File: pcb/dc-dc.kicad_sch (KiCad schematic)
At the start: 30 parts

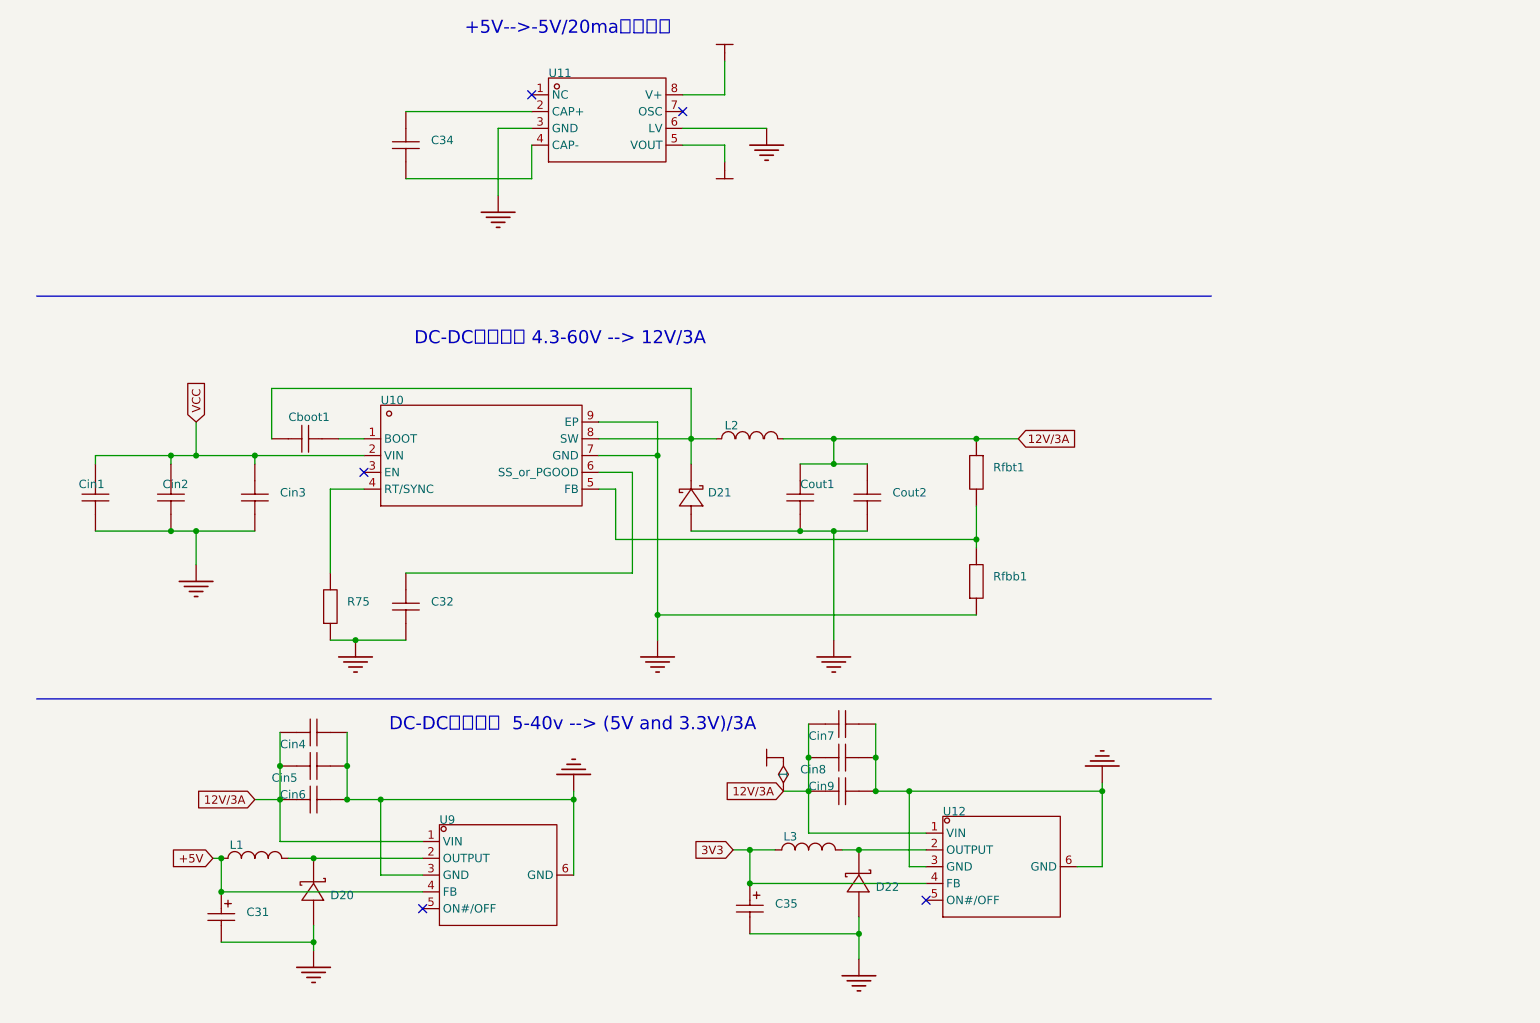
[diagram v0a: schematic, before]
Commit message: feat: update
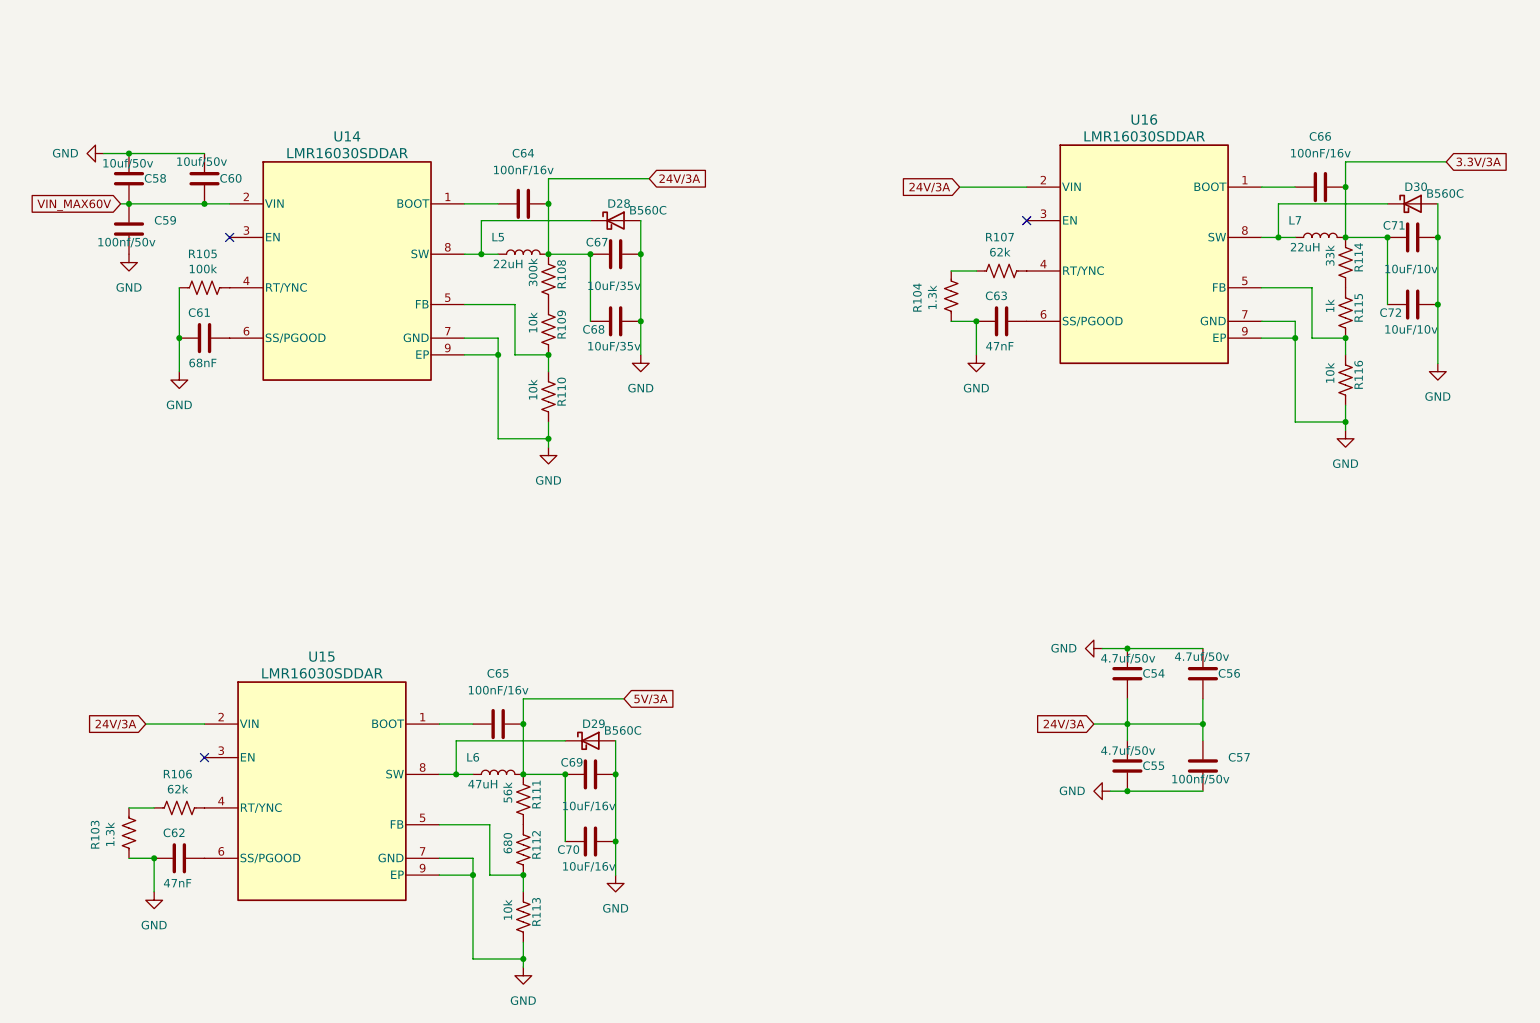
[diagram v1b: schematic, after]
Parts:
- removed 1: ~, ProDoc_CAN-easyedapro:, symbol ProDoc_CAN-easyedapro:Short-Symbol
- removed C31: 220uF, ProDoc_CAN-easyedapro:CASE-D_7343, symbol ProDoc_CAN-easyedapro:TAJD227K010RNJ
- removed C32: 33uF/25V, ProDoc_CAN-easyedapro:C0603, symbol ProDoc_CAN-easyedapro:CapAcitance
- removed C34: 47uF/25V, ProDoc_CAN-easyedapro:C0603, symbol ProDoc_CAN-easyedapro:CapAcitance
- removed C35: 330uF, ProDoc_CAN-easyedapro:CAP-SMD_L6.0-W3.2-R-RD, symbol ProDoc_CAN-easyedapro:TAJC337K006RNJ
- removed Cboot1: 0.1uF/50V, ProDoc_CAN-easyedapro:C0603, symbol ProDoc_CAN-easyedapro:CapAcitance
- removed Cin1, Cin6, Cin9: 0.1uF/100V, ProDoc_CAN-easyedapro:C0603, symbol ProDoc_CAN-easyedapro:CapAcitance
- removed Cin2, Cin3, Cin4, Cin5, Cin7, Cin8: 2.2uF/100V, ProDoc_CAN-easyedapro:C0603, symbol ProDoc_CAN-easyedapro:CapAcitance
- removed Cout1, Cout2: 47uF/50V, ProDoc_CAN-easyedapro:C0603, symbol ProDoc_CAN-easyedapro:CapAcitance
- removed D20, D22: ~, ProDoc_CAN-easyedapro:SMC_L7.5-W5.8-LS8.3-RD, symbol ProDoc_CAN-easyedapro:SS53C
- removed D21: ~, ProDoc_CAN-easyedapro:SMC_L6.9-W5.9-LS7.9-RD, symbol ProDoc_CAN-easyedapro:SS510SMC
- removed L1, L3: 33uH, ProDoc_CAN-easyedapro:IND-SMD_L11.5-W10.0_FXL1040, symbol ProDoc_CAN-easyedapro:FXL1040-330-M
- removed L2: 8.2uH, ProDoc_CAN-easyedapro:IND-SMD_L7.0-W6.6_FXL0630, symbol ProDoc_CAN-easyedapro:FXL0630-8R2-M
- removed R75: 50k, ProDoc_CAN-easyedapro:R0603, symbol ProDoc_CAN-easyedapro:电阻
- removed Rfbb1: 6.67k, ProDoc_CAN-easyedapro:R0603, symbol ProDoc_CAN-easyedapro:电阻
- removed Rfbt1: 100k, ProDoc_CAN-easyedapro:R0603, symbol ProDoc_CAN-easyedapro:电阻
- removed U10: ~, ProDoc_CAN-easyedapro:SO-8_L4.9-W3.9-P1.27-LS6.0-BL-EP, symbol ProDoc_CAN-easyedapro:LMR16030SDDAR
- removed U11: ~, ProDoc_CAN-easyedapro:SOP-8_L4.9-W3.9-P1.27-LS6.0-BL, symbol ProDoc_CAN-easyedapro:HT7660ARZ
- removed U12: ~, ProDoc_CAN-easyedapro:TO-263-5_L10.1-W8.7-P1.70-LS14.4-BR, symbol ProDoc_CAN-easyedapro:LM2596S-3.3/TR
- removed U9: ~, ProDoc_CAN-easyedapro:TO-263-5_L10.2-W8.6-P1.70-LS14.4-TL, symbol ProDoc_CAN-easyedapro:LM2596S-5.0/TR
- added C54, C55, C56: 4.7uf/50v, Capacitor_SMD:C_1206_3216Metric, symbol Device:C
- added C57, C59: 100nf/50v, Capacitor_SMD:C_0603_1608Metric, symbol Device:C
- added C58, C60: 10uf/50v, Capacitor_SMD:C_1210_3225Metric, symbol Device:C
- added C61: 68nF, Capacitor_SMD:C_0603_1608Metric, symbol Device:C
- added C62, C63: 47nF, Capacitor_SMD:C_0603_1608Metric, symbol Device:C
- added C64, C65, C66: 100nF/16v, Capacitor_SMD:C_0603_1608Metric, symbol Device:C
- added C67, C68: 10uF/35v, Capacitor_SMD:C_1210_3225Metric, symbol Device:C
- added C69, C70: 10uF/16v, Capacitor_SMD:C_1210_3225Metric, symbol Device:C
- added C71, C72: 10uF/10v, Capacitor_SMD:C_0603_1608Metric, symbol Device:C
- added D28, D29, D30: B560C, Diode_SMD:D_SMC, symbol Device:D_Schottky
- added L5, L7: 22uH, Inductor_SMD:L_TDK_SLF12565, symbol Device:L
- added L6: 47uH, Inductor_SMD:L_TDK_SLF12565, symbol Device:L
- added R103, R104: 1.3k, Resistor_SMD:R_0603_1608Metric, symbol Device:R_US
- added R105: 100k, Resistor_SMD:R_0603_1608Metric, symbol Device:R_US
- added R106, R107: 62k, Resistor_SMD:R_0603_1608Metric, symbol Device:R_US
- added R108: 300k, Resistor_SMD:R_0603_1608Metric, symbol Device:R_US
- added R109, R110, R113, R116: 10k, Resistor_SMD:R_0603_1608Metric, symbol Device:R_US
- added R111: 56k, Resistor_SMD:R_0603_1608Metric, symbol Device:R_US
- added R112: 680, Resistor_SMD:R_0603_1608Metric, symbol Device:R_US
- added R114: 33k, Resistor_SMD:R_0603_1608Metric, symbol Device:R_US
- added R115: 1k, Resistor_SMD:R_0603_1608Metric, symbol Device:R_US
- added U14, U15, U16: LMR16030SDDAR, Package_SO:TI_SO-PowerPAD-8_ThermalVias, symbol 2025-01-08_11-11-09:LMR16030SDDAR
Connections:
- new net: D29.1 (K), L6.1, U15.8 (SW)
- new net: R104.1, R107.2
- new net: C63.1, U16.6 (SS/PGOOD)
- new net: C61.1, U14.6 (SS/PGOOD)
- new net: C66.2, U16.1 (BOOT)
- new net: C64.2, U14.1 (BOOT)
- new net: R105.1, U14.4 (RT/YNC)
- new net: R109.2, R110.1, U14.5 (FB)
- new net: D28.1 (K), L5.1, U14.8 (SW)
- new net: C65.2, U15.1 (BOOT)
- new net: R111.2, R112.1
- new net: R112.2, R113.1, U15.5 (FB)
- new net: R114.2, R115.1
- new net: R115.2, R116.1, U16.5 (FB)
- new net: C62.1, U15.6 (SS/PGOOD)
- new net: R108.2, R109.1
- new net: R106.1, U15.4 (RT/YNC)
- new net: D30.1 (K), L7.1, U16.8 (SW)
- new net: R107.1, U16.4 (RT/YNC)
- new net: R103.1, R106.2
- new net 24V/3A: C54.1, C55.2, C56.2, C57.1, C64.1, C67.1, C68.2, L5.2, R108.1, U15.2 (VIN), U16.2 (VIN)
- new net 3.3V/3A: C66.1, C71.1, C72.2, L7.2, R114.1
- new net 5V/3A: C65.1, C69.1, C70.2, L6.2, R111.1
- new net GND: C54.2, C55.1, C56.1, C57.2, C58.2, C59.2, C60.1, C61.2, C62.2, C63.2, C67.2, C68.1, C69.2, C70.1, C71.2, C72.1, D28.2 (A), D29.2 (A), D30.2 (A), R103.2, R104.2, R105.2, R110.2, R113.2, R116.2, U14.7 (GND), U14.9 (EP), U15.7 (GND), U15.9 (EP), U16.7 (GND), U16.9 (EP)
- new net VIN_MAX60V: C58.1, C59.1, C60.2, U14.2 (VIN)
- no-connect marks 5 -> 3
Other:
- note removed: "+5V-->-5V/20ma电压翻转"
- note removed: "DC-DC降压模块 4.3-60V --> 12V/3A"
- note removed: "DC-DC降压模块 5-40v --> (5V and 3.3V)/3A"
